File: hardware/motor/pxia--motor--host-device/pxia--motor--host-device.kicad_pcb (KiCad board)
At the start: 2 copper layers, 35.7 x 45.8 mm, 5 parts, among them J1 RJ45, U1 Teensy4.0, U2 max3490eesa+T

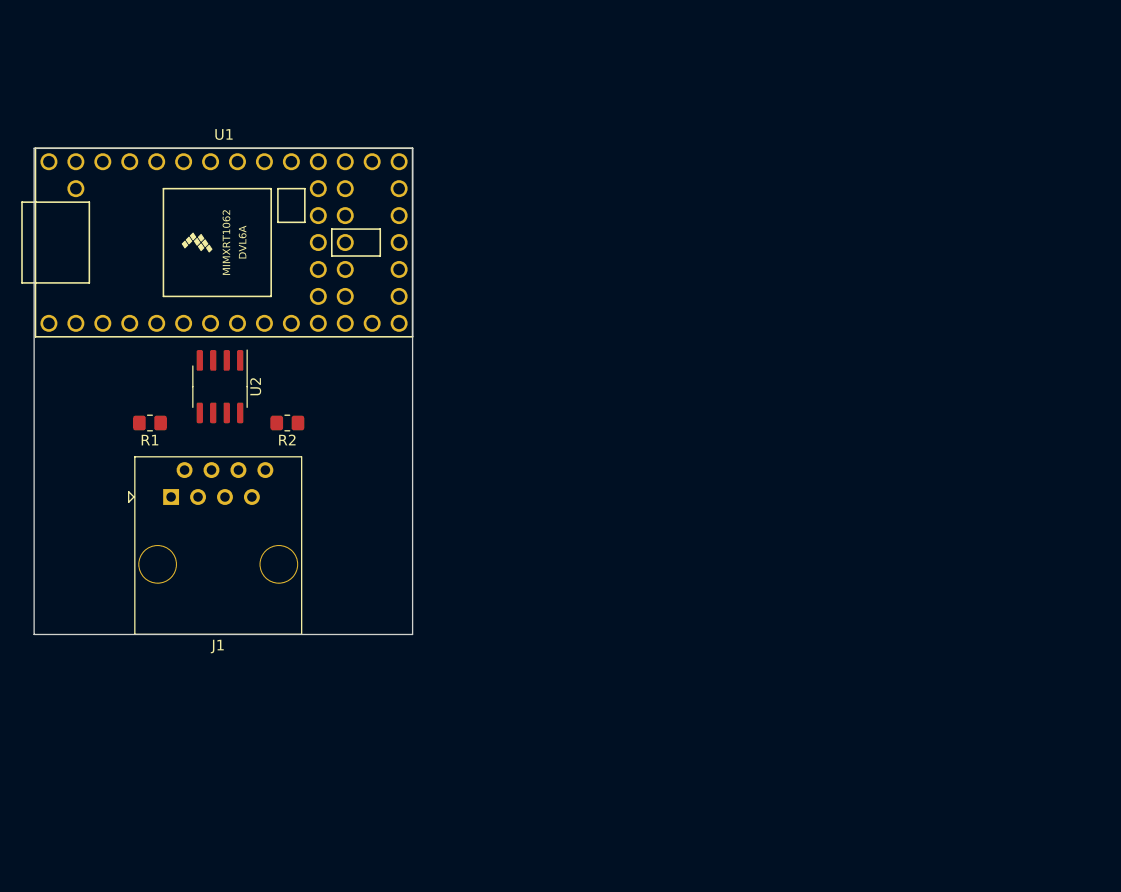
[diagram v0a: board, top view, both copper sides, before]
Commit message: finished schematics and most of pcb layout
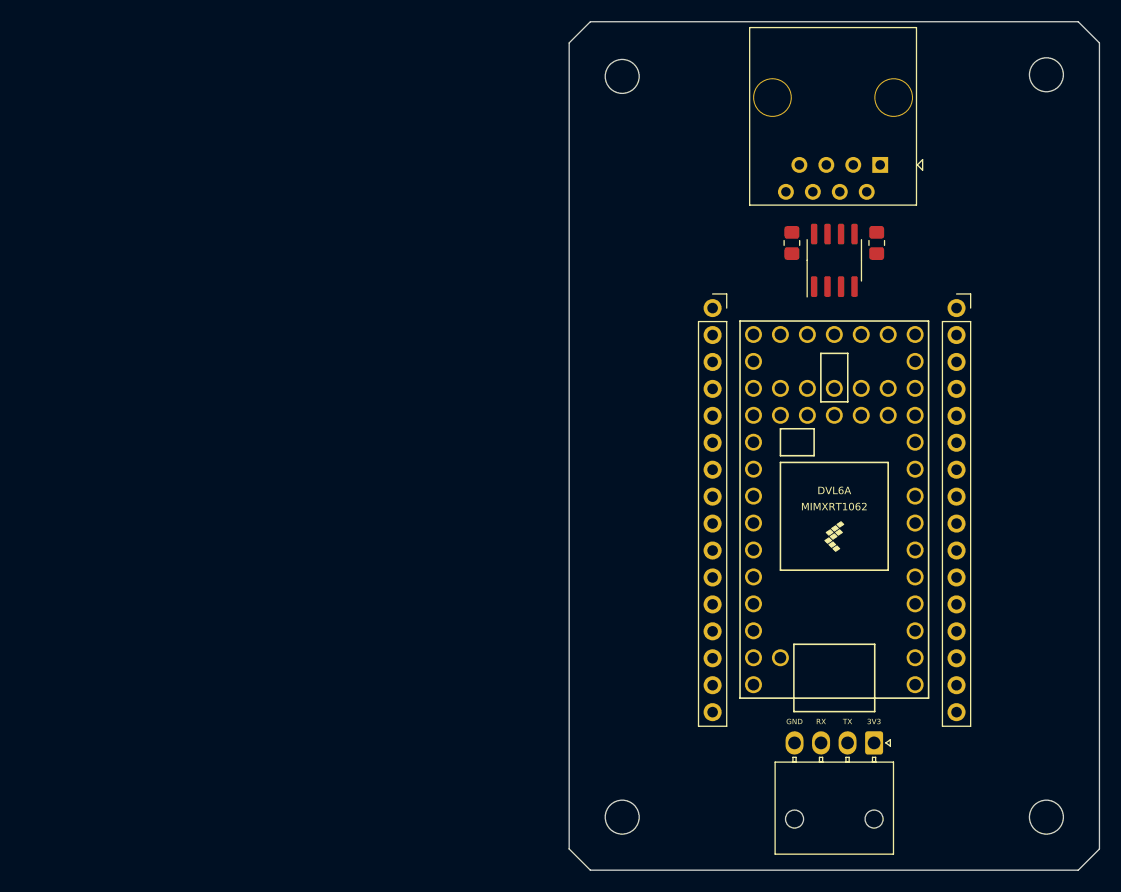
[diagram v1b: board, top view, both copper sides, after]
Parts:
- added H1: M3, MountingHole:MountingHole_3.2mm_M3, F.Cu at (130.0, 60.2)
- added H2: M3, MountingHole:MountingHole_3.2mm_M3, F.Cu at (170.0, 60.0)
- added H3: M3, MountingHole:MountingHole_3.2mm_M3, F.Cu at (170.0, 130.0)
- added H4: M3, MountingHole:MountingHole_3.2mm_M3, F.Cu at (130.0, 130.0)
- added J2: Lolin D32 Pro 2.0.0 (ESP32) PIN01–16, Connector_PinSocket_2.54mm:PinSocket_1x16_P2.54mm_Vertical, F.Cu at (138.5, 82.0)
- added J3: GENERIC_UART, Connector_Molex:Molex_Nano-Fit_105313-xx04_1x04_P2.50mm_Horizontal, F.Cu at (153.8, 123.0)
- added J4: Lolin D32 Pro 2.0.0 (ESP32) PIN17–32, Connector_PinSocket_2.54mm:PinSocket_1x16_P2.54mm_Vertical, F.Cu at (161.5, 82.0)
- moved J1 73.8 mm to (154.3, 68.5), turned to 180 degrees
- moved R1 62.9 mm to (146.0, 75.9), turned to 90 degrees
- moved U1 62.8 mm to (150.0, 101.0), turned to 90 degrees
- moved U2 59.1 mm to (150.0, 77.5), turned to 90 degrees
- moved Re 58.1 mm to (154.0, 75.9), turned to -90 degrees
- renumbered R2 to Re
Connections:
- net /MCU_RX renamed /IO13
- net /MCU_TX renamed /IO14/T-CS
- J1 pad 3: GND -> unconnected-(J1-Pad3)
- J1 pad 4: GND -> unconnected-(J1-Pad3)
- J1 pad 5: GND -> unconnected-(J1-Pad3)
- J1 pad 6: GND -> unconnected-(J1-Pad3)
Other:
- board size 35.7 x 45.8 mm -> 50 x 80 mm
- board text added: "3V3"
- board text added: "GND"
- board text added: "RX"
- board text added: "TX"
- board text removed: "@TODO(FIND CORRECT FOOTPRINT ON JLCPCB)"
